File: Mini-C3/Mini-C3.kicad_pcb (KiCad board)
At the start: 2 copper layers, 84.8 x 23.5 mm, 21 parts, among them J1 TB_1X2, J10 Sensor1, J11 Sensor1, J12 Sensor1, J2 Sensor1, J3 Sensor1, J4 MotorB, J5 MotorA, J6 Sensor1, J7 Sensor1, J8 Sensor1, J9 Sensor1, SW1 SW_Push, U1 Driver Module, U2 ESP32-C3_SUPERMINI, U3 Mini360

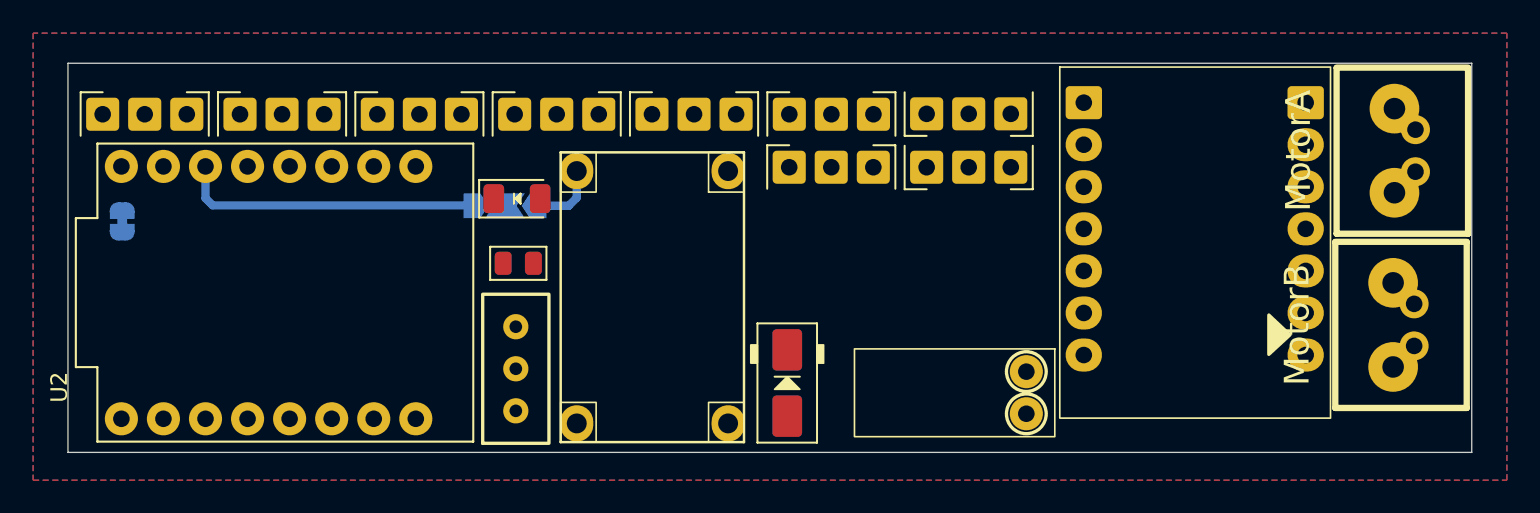
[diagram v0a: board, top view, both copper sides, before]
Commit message: PCB almost there
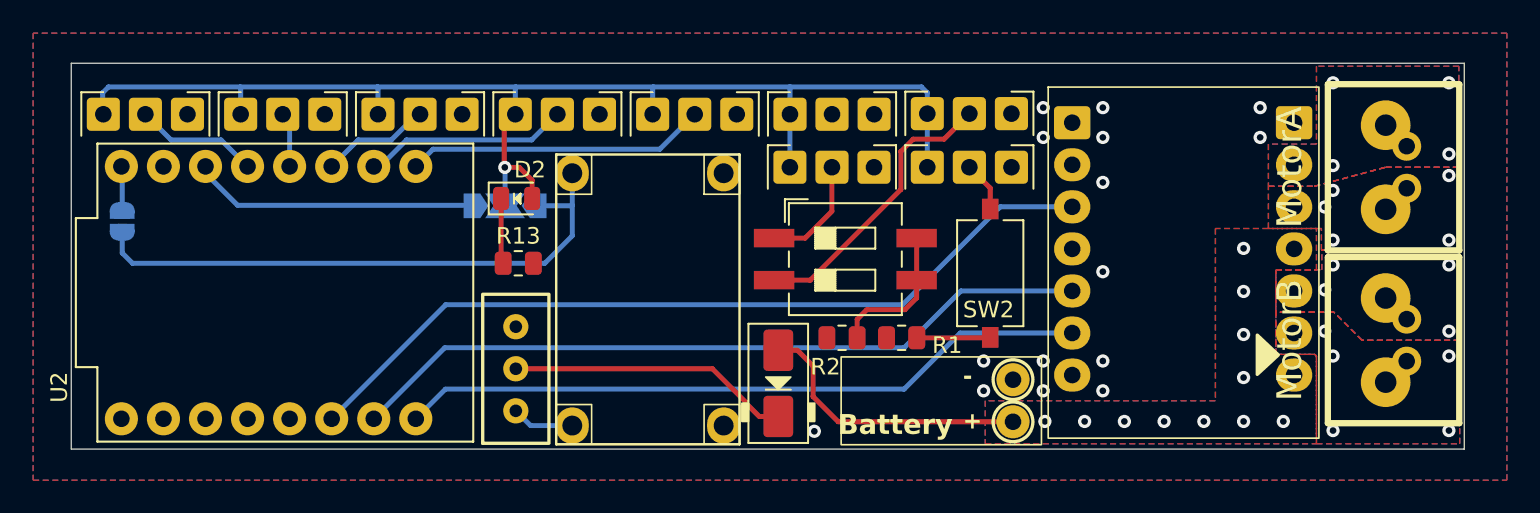
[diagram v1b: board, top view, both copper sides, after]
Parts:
- added R1: 100, Resistor_SMD:R_0805_2012Metric, F.Cu at (158.4, 96.4)
- added R2: 100, Resistor_SMD:R_0805_2012Metric, F.Cu at (154.8, 96.4)
- added SW2: SW_Push, Button_Switch_SMD:SW_Tactile_SPST_NO_Straight_CK_PTS636Sx25SMTRLFS, F.Cu at (163.8, 92.5)
- added SW3: SW_DIP_x02, Button_Switch_SMD:SW_DIP_SPSTx02_Slide_6.7x6.64mm_W8.61mm_P2.54mm_LowProfile, F.Cu at (155.1, 91.7)
- D2: footprint MixLib:LED_1206_3216Metric -> MixLib:LED_0805_2012Metric
- JP7: footprint Jumper:SolderJumper-2_P1.3mm_Bridged_RoundedPad1.0x1.5mm -> Jumper:SolderJumper-2_P1.3mm_Open_RoundedPad1.0x1.5mm
- R13: footprint PCM_Resistor_SMD_AKL:R_0805_2012Metric -> Resistor_SMD:R_0805_2012Metric
- moved J11 1.40 mm to (162.5, 86.8), turned to 180 degrees
- moved U1 1.40 mm to (175.3, 91.8)
- moved J12 1.39 mm to (162.5, 83.6), turned to 180 degrees
- moved J5 1.13 mm to (187.7, 86.1)
- moved J4 1.02 mm to (187.7, 96.5)
- moved J1 0.94 mm to (160.4, 100.2)
- moved D1 0.54 mm to (151.0, 99.2), turned to 90 degrees
- moved U3 0.30 mm to (143.1, 94.1)
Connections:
- J10 pad 1: /Pin5 -> GND
- J10 pad 2: GND -> /Pin0
- J11 pad 1: /Pin7 -> GND
- J11 pad 2: GND -> /Pin7
- J12 pad 1: /Pin8 -> GND
- J12 pad 2: GND -> /Pin8
- J2 pad 1: /Pin0 -> GND
- J2 pad 2: GND -> /Pin5
- J3 pad 1: /Pin6 -> GND
- J3 pad 2: GND -> /Pin6
- J6 pad 2: unconnected-(J6-Pin_2-Pad2) -> /Pin1
- J7 pad 1: /Pin2 -> GND
- J7 pad 2: GND -> /Pin2
- J8 pad 1: /Pin3 -> GND
- J8 pad 2: GND -> /Pin3
- J9 pad 1: /Pin4 -> GND
- J9 pad 2: GND -> /Pin4
- SW1 pad 1: (no net) -> Net-(U3-IN)
- SW1 pad 2: Net-(U3-IN) -> Net-(D1-K)
- SW1 pad 3: Net-(D1-K) -> (no net)
- U2 pad 1: GND -> /Pin1
- U2 pad 10: /IN_A2 -> /IN_B1
- U2 pad 20: /IN_B1 -> /IN_A2
- U2 pad 21: /IN_B2 -> /IN_A1
- U2 pad 9: /IN_A1 -> /IN_B2
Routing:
- net /Vcc: track 0.00 -> 76.3 mm, vias 0 -> 1
- net /IN_B1: track 0.00 -> 50.0 mm
- net /IN_A2: track 0.00 -> 45.4 mm
- net /IN_A1: track 0.00 -> 41.8 mm
- net +5V: track 4.14 -> 35.2 mm
- net /Pin0: track 0.00 -> 18.1 mm
- net /Pin8: track 0.00 -> 17.3 mm
- net Net-(D1-K): track 0.00 -> 17.1 mm
- net /VM: track 0.00 -> 17.0 mm, vias 0 -> 11
- net /Pin1: track 0.00 -> 12.4 mm
- net Net-(R2-Pad2): track 0.00 -> 8.86 mm
- net /Pin4: track 0.00 -> 7.47 mm
- net /Pin6: track 0.00 -> 6.83 mm
- net /Pin2: track 0.00 -> 6.64 mm
- net Net-(R1-Pad1): track 0.00 -> 4.45 mm
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- added copper zone on B.Cu, net /OUT_A1
- added copper zone on F.Cu, net /OUT_A1
- added copper zone on B.Cu, net /OUT_A2
- added copper zone on F.Cu, net /OUT_A2
- added copper zone on B.Cu, net /OUT_B1
- added copper zone on F.Cu, net /OUT_B1
- added copper zone on B.Cu, net /OUT_B2
- added copper zone on F.Cu, net /OUT_B2
- added copper zone on B.Cu, net /VM
- added copper zone on F.Cu, net /VM
- added copper zone on B.Cu, net GND
- added copper zone on F.Cu, net GND
- removed copper zone on B.Cu, net /Vcc
- removed copper zone on F.Cu, net /Vcc
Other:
- board size 84.8 x 23.5 mm -> 84.1 x 23.3 mm
- board text added: "+"
- board text added: "-"
- board text added: "Battery"
